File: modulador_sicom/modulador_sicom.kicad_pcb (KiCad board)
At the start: 2 copper layers, 50 x 50 mm, 28 parts, among them J1 POWER, U1 MC1496D, U2 L7812

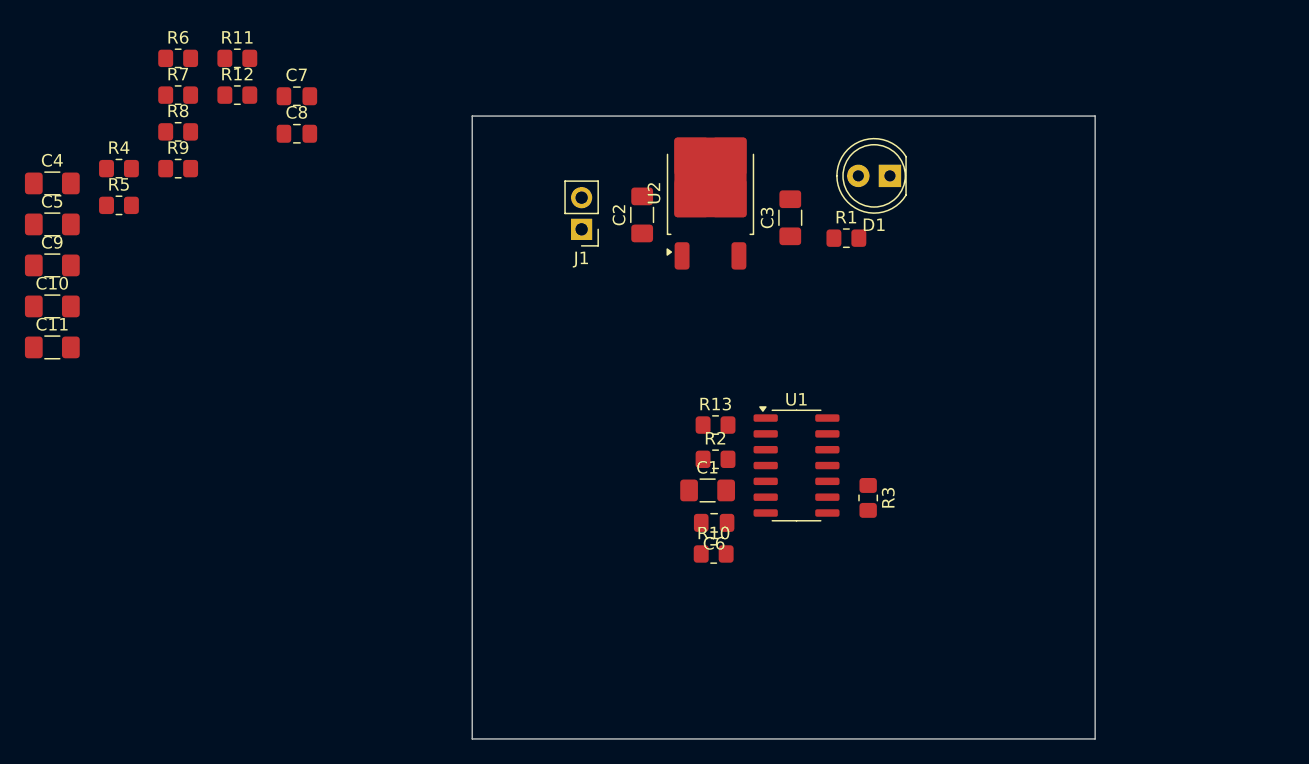
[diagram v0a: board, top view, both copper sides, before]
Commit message: Update latest changes.
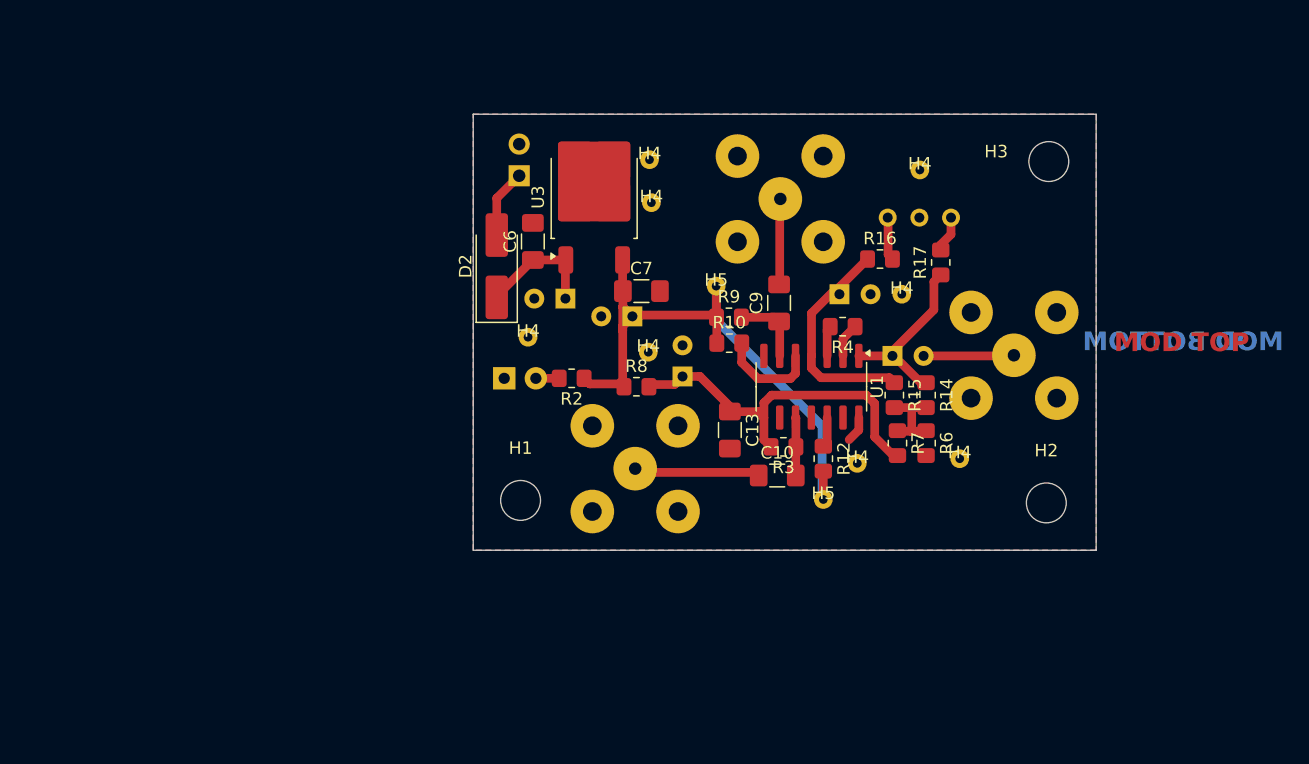
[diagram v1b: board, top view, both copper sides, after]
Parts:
- removed C11, C2, C3: 100n, Inductor_SMD:L_1206_3216Metric_Pad1.42x1.75mm_HandSolder
- removed D1: LED, LED_THT:LED_D5.0mm
- removed J1: POWER, Connector_PinHeader_2.54mm:PinHeader_1x02_P2.54mm_Vertical
- removed R1, R11, R5: 1k, Resistor_SMD:R_0805_2012Metric_Pad1.20x1.40mm_HandSolder
- removed R13: 51, Resistor_SMD:R_0805_2012Metric_Pad1.20x1.40mm_HandSolder
- removed U2: L7812, Package_TO_SOT_SMD:TO-252-2
- added C12: 25u, Capacitor_THT:CP_Radial_D5.0mm_P2.50mm, B.Cu at (154.6, 95.3)
- added C13: 100n, Inductor_SMD:L_1206_3216Metric_Pad1.42x1.75mm_HandSolder, F.Cu at (158.4, 99.7)
- added D2: 1N4007, Diode_SMD:D_SMA_Handsoldering, F.Cu at (139.7, 86.5)
- added D3: LED, LED_THT:LED_D5.0mm, B.Cu at (140.3, 95.5)
- added H1: MountingHole, MountingHole:MountingHole_3.2mm_M3, F.Cu at (141.6, 105.3)
- added H2: MountingHole, MountingHole:MountingHole_3.2mm_M3, F.Cu at (183.8, 105.5)
- added H3: MountingHole, MountingHole:MountingHole_3.2mm_M3, F.Cu at (184.0, 78.1)
- added H4: ~, via:Via_0.7x1.5, F.Cu at (151.9, 78.0)
- added H4: ~, via:Via_0.7x1.5, F.Cu at (152.1, 81.4)
- added H4: ~, via:Via_0.7x1.5, F.Cu at (142.2, 92.2)
- added H4: ~, via:Via_0.7x1.5, F.Cu at (151.8, 93.4)
- added H4: ~, via:Via_0.7x1.5, F.Cu at (173.7, 78.8)
- added H4: ~, via:Via_0.7x1.5, F.Cu at (168.6, 102.3)
- added H4: ~, via:Via_0.7x1.5, F.Cu at (176.8, 102.0)
- added H4: ~, via:Via_0.7x1.5, F.Cu at (172.2, 88.8)
- added H5: ~, via:Via_0.7x1.5, F.Cu at (157.3, 88.1)
- added H5: ~, via:Via_0.7x1.5, F.Cu at (165.9, 105.2)
- added J2: OUTPUT, connector:BNC_TEConnectivity_413969-2, B.Cu at (162.4, 81.1)
- added J3: CARRIER_IN, connector:BNC_TEConnectivity_413969-2, B.Cu at (150.8, 102.8)
- added J4: MODULATING, connector:BNC_TEConnectivity_413969-2, B.Cu at (181.2, 93.7)
- added J5: POWER, Connector_PinHeader_2.54mm:PinHeader_1x02_P2.54mm_Vertical, B.Cu at (141.5, 79.2)
- added R14: 100, Resistor_SMD:R_0805_2012Metric_Pad1.20x1.40mm_HandSolder, F.Cu at (174.2, 96.8)
- added R15: 100, Resistor_SMD:R_0805_2012Metric_Pad1.20x1.40mm_HandSolder, F.Cu at (171.6, 96.8)
- added R16: 10k, Resistor_SMD:R_0805_2012Metric_Pad1.20x1.40mm_HandSolder, F.Cu at (170.4, 85.9)
- added R17: 10k, Resistor_SMD:R_0805_2012Metric_Pad1.20x1.40mm_HandSolder, F.Cu at (175.3, 86.2)
- added RV1: 10k, Potentiometer_THT:Potentiometer_Bourns_3296W_Vertical, B.Cu at (176.2, 82.6)
- added U3: L7812, Package_TO_SOT_SMD:TO-252-2, F.Cu at (147.5, 81.0)
- C1: value 100n -> 25u; footprint Inductor_SMD:L_1206_3216Metric_Pad1.42x1.75mm_HandSolder -> Capacitor_THT:CP_Radial_D5.0mm_P2.50mm; moved to B.Cu
- C4, C5: value 100n -> 10u; footprint Inductor_SMD:L_1206_3216Metric_Pad1.42x1.75mm_HandSolder -> Capacitor_THT:CP_Radial_D5.0mm_P2.50mm; moved to B.Cu
- C6, C7: value 4.7n -> 100n; footprint Capacitor_SMD:C_0805_2012Metric_Pad1.18x1.45mm_HandSolder -> Inductor_SMD:L_1206_3216Metric_Pad1.42x1.75mm_HandSolder
- C8: value 4.7n -> 10u; footprint Capacitor_SMD:C_0805_2012Metric_Pad1.18x1.45mm_HandSolder -> Capacitor_THT:CP_Radial_D5.0mm_P2.50mm; moved to B.Cu
- R2: value 51 -> 1k
- moved C4 68.8 mm to (171.4, 93.7)
- moved R6 67.5 mm to (174.2, 100.7), turned to -90 degrees
- moved R7 64.1 mm to (171.8, 100.7), turned to -90 degrees
- moved C10 59.7 mm to (162.2, 103.3)
- moved R4 59.5 mm to (167.4, 91.3), turned to 180 degrees
- moved C9 58.4 mm to (162.3, 89.5), turned to 90 degrees
- moved R12 55.4 mm to (165.9, 102.0), turned to -90 degrees
- moved R9 45.8 mm to (158.3, 90.6)
- moved R8 42.1 mm to (150.9, 96.2)
- moved C5 41.6 mm to (145.2, 89.1), turned to 180 degrees
- moved C7 31.8 mm to (151.3, 88.5)
- moved C8 30.7 mm to (150.6, 90.5), turned to 180 degrees
- moved C6 26.9 mm to (142.6, 84.5), turned to 90 degrees
- moved C1 19.0 mm to (167.2, 88.8)
- moved R10 17.0 mm to (158.3, 92.7)
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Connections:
- net Net-(U1-CARRIER_IN) renamed /CARRIER_A
- C10 pad 1: Net-(J3-In) -> /CARRIER
- C4 pad 1: Net-(C4-Pad1) -> /MOD_A
- C4 pad 2: GND -> /MOD
- C5 pad 1: Net-(C5-Pad1) -> /V_IN
- C6 pad 1: Net-(C6-Pad1) -> /V_IN
- C7 pad 1: Net-(C7-Pad1) -> +12V
- C8 pad 1: Net-(C8-Pad1) -> +12V
- C9 pad 1: Net-(C8-Pad1) -> /OUT_A
- C9 pad 2: Net-(J2-In) -> /OUT
- R12 pad 1: +12V -> Net-(R12-Pad1)
- R12 pad 2: Net-(C7-Pad1) -> +12V
- R2 pad 1: Net-(R13-Pad1) -> +12V
- R2 pad 2: Net-(U1-GAIN_ADJ_2) -> Net-(D3-A)
- R4 pad 1: Net-(C4-Pad1) -> Net-(U1-GAIN_ADJ)
- R4 pad 2: Net-(U1-SIG_IN) -> Net-(U1-GAIN_ADJ_2)
- R6 pad 1: GND -> Net-(R14-Pad2)
- R6 pad 2: Net-(C4-Pad1) -> GND
- R7 pad 1: Net-(C4-Pad1) -> Net-(R14-Pad2)
- R7 pad 2: Net-(C5-Pad1) -> Net-(U1-IN_CARRIER)
- R8 pad 2: Net-(C5-Pad1) -> Net-(U1-IN_CARRIER)
- R9 pad 2: Net-(C6-Pad1) -> /OUT_A
- U1 pad 1: Net-(U1-SIG_IN_2) -> /MOD_A
- U1 pad 12: Net-(C7-Pad1) -> Net-(R12-Pad1)
- U1 pad 6: Net-(C6-Pad1) -> /OUT_A
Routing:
- net +12V: track 0.00 -> 50.7 mm
- net Net-(U1-IN_CARRIER): track 0.00 -> 29.5 mm
- net Net-(U1-SIG_IN): track 0.00 -> 19.0 mm
- net /MOD_A: track 0.00 -> 14.4 mm
- net /CARRIER: track 0.00 -> 10.1 mm
- net /V_IN: track 0.00 -> 9.95 mm
- net Net-(U1-BIAS): track 0.00 -> 7.99 mm
- net /MOD: track 0.00 -> 7.27 mm
- net /OUT: track 0.00 -> 6.90 mm
- net Net-(R14-Pad2): track 0.00 -> 6.81 mm
- net /OUT_A: track 0.00 -> 5.95 mm
- net Net-(D2-A): track 0.00 -> 5.51 mm
- net /CARRIER_A: track 0.00 -> 4.67 mm
- net Net-(R16-Pad2): track 0.00 -> 3.48 mm
- net Net-(R17-Pad2): track 0.00 -> 2.94 mm
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- added copper zone on B.Cu, net GND
- added copper zone on F.Cu, net GND
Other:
- board size 50 x 50 mm -> 50 x 35 mm
- board text added: "MOD BOTTOM"
- board text added: "MOD TOP"
